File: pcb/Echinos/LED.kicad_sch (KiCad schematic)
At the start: 14 parts

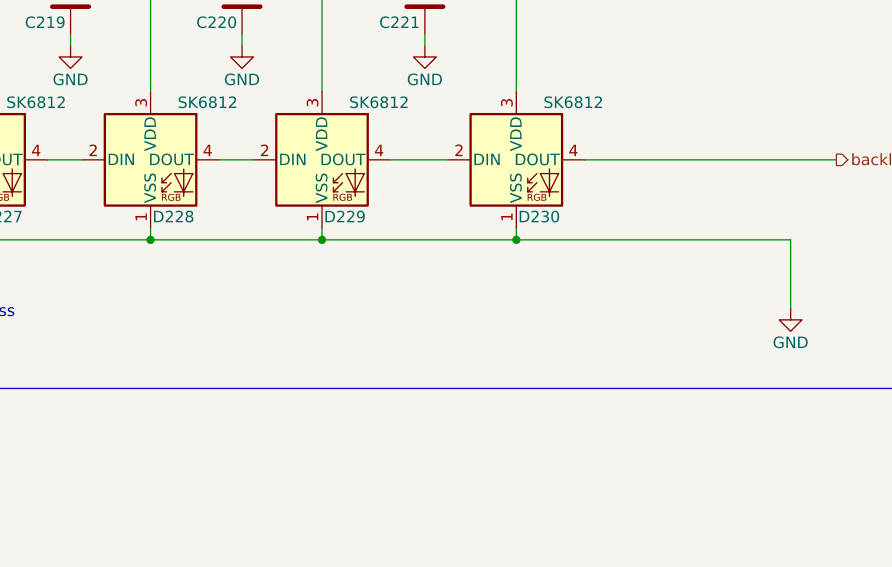
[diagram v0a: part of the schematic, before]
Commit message: 🚀 [PCB] - Board RP2040 sent in production.
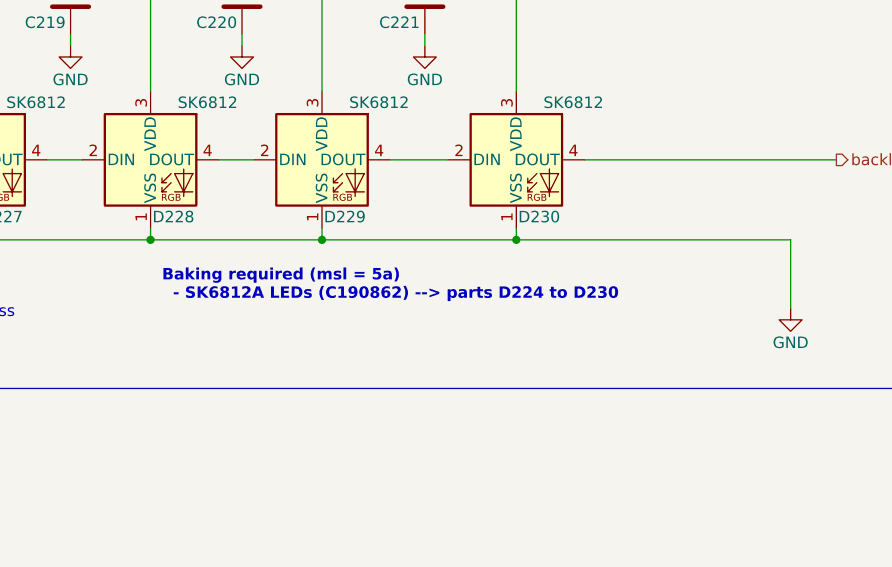
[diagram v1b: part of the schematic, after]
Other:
- note added: "Baking required (msl = 5a) - SK6812A LEDs (C190862) --> parts D224 to D230"
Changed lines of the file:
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@@
+		)
+	)
+	(text "Baking required (msl = 5a)\n  - SK6812A LEDs (C190862) --> parts D224 to D230"
+		(exclude_from_sim no)
+		(at 148.59 69.215 0)
+		(effects
+			(font
+				(size 1.27 1.27)
+				(thickness 0.254)
+				(bold yes)
+			)
+			(justify left)
 		)
 	)
